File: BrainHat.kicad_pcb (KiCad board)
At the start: 2 copper layers, 86 x 51.2 mm, 47 parts, among them J1 Power, J2 Output, J3 Electrodes, J4 Status, U1 AD8232, U2 ADS1115IDGS, U3 TS5A3159ADBVR, U4 SN74LV1T34DBV, U5 SN74LV1T34DBV

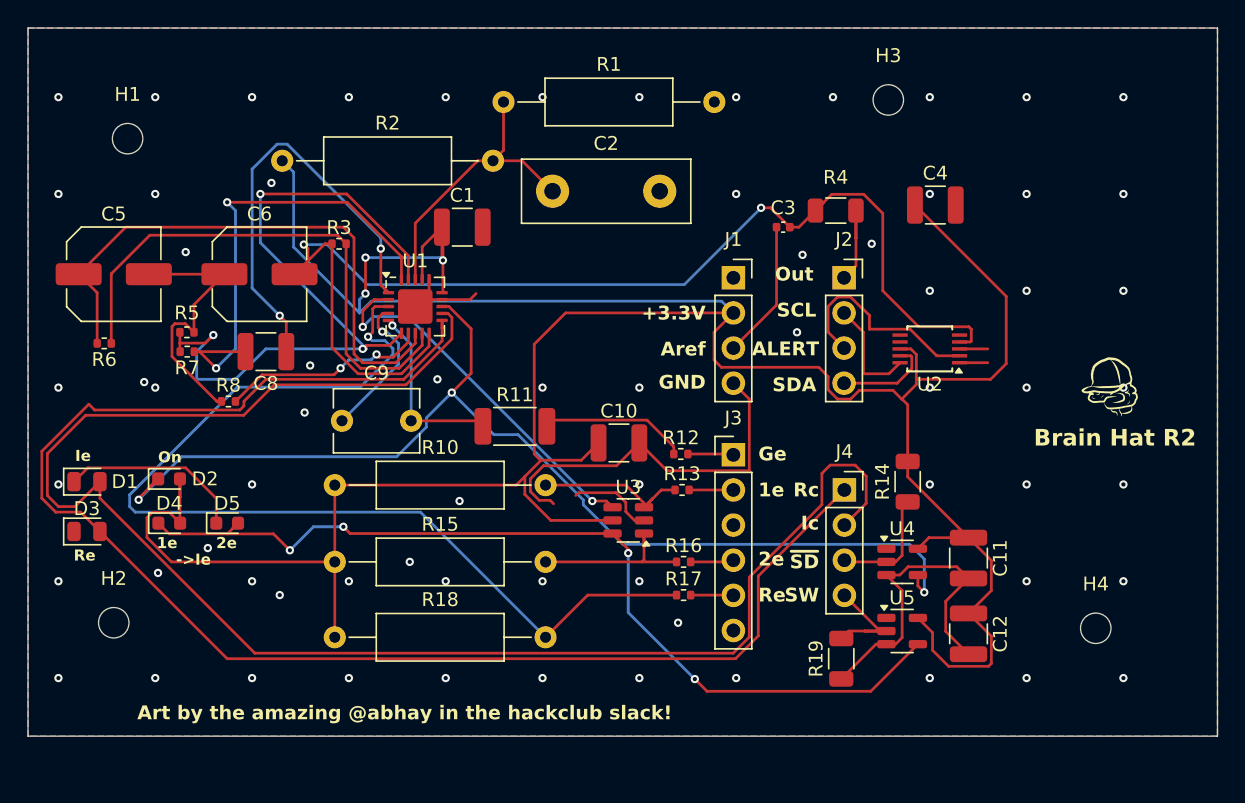
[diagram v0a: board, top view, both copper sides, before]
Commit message: Redid PCB again
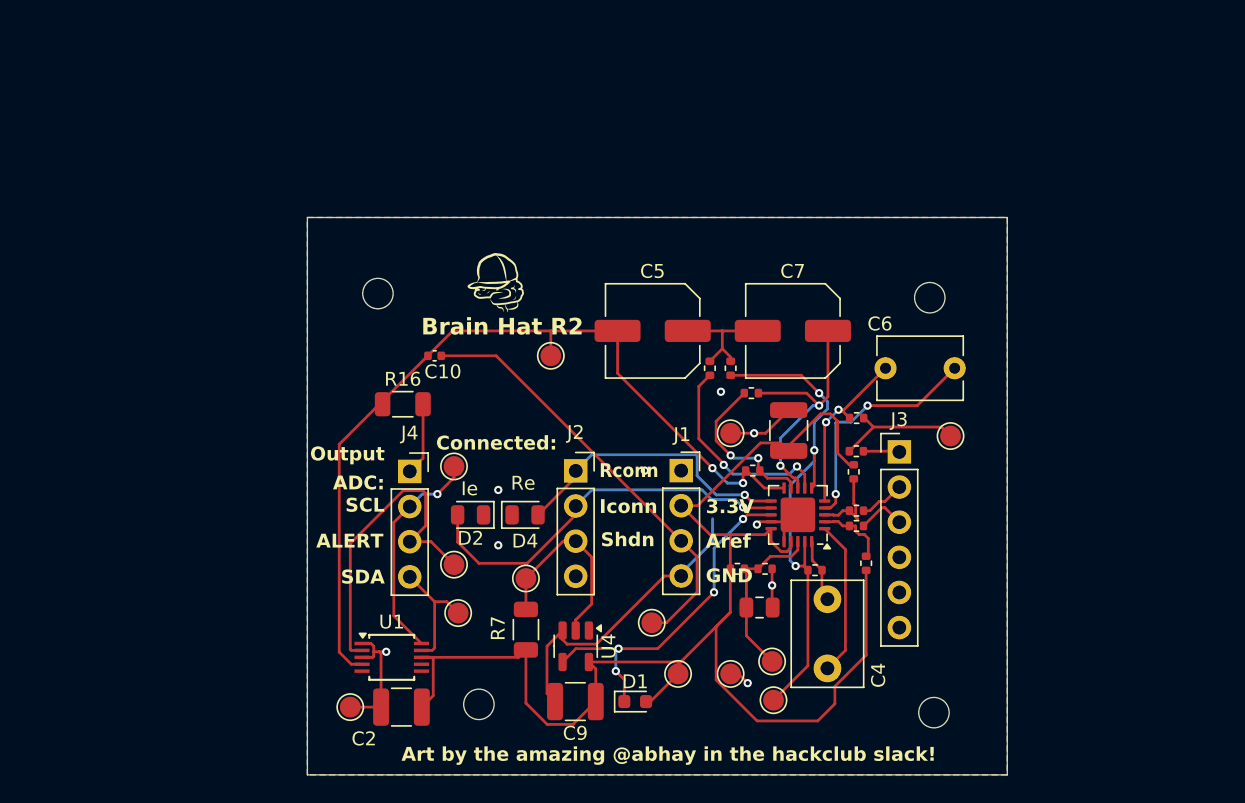
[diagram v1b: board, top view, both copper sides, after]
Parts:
- removed C11, C12, C8: 100nF, Capacitor_SMD:C_1210_3225Metric
- removed D3: XL-2012UWC, LED_SMD:LED_0805_2012Metric
- removed D5: XL-1608UGC-04, LED_SMD:LED_0603_1608Metric
- removed R17: 330k, Resistor_SMD:R_0402_1005Metric
- removed R18: 10M±1%, Resistor_THT:R_Axial_DIN0309_L9.0mm_D3.2mm_P15.24mm_Horizontal
- removed R19: 10k, Resistor_SMD:R_1206_3216Metric
- removed U3: TS5A3159ADBVR, Package_TO_SOT_SMD:SOT-23-6
- removed U5: SN74LV1T34DBV, Package_TO_SOT_SMD:SOT-23-5
- added C7: 220uF, Capacitor_SMD:C_Elec_6.3x5.4, F.Cu at (186.1, 72.9)
- added TP1: TestPoint, TestPoint:TestPoint_Pad_D1.5mm, F.Cu at (181.6, 80.3)
- added TP10: TestPoint, TestPoint:TestPoint_Pad_D1.5mm, F.Cu at (154.1, 100.1)
- added TP12: TestPoint, TestPoint:TestPoint_Pad_D1.5mm, F.Cu at (166.8, 90.8)
- added TP13: TestPoint, TestPoint:TestPoint_Pad_D1.5mm, F.Cu at (197.5, 80.5)
- added TP16: TestPoint, TestPoint:TestPoint_Pad_D1.5mm, F.Cu at (168.6, 74.7)
- added TP2: TestPoint, TestPoint:TestPoint_Pad_D1.5mm, F.Cu at (177.8, 97.7)
- added TP3: TestPoint, TestPoint:TestPoint_Pad_D1.5mm, F.Cu at (175.9, 94.0)
- added TP4: TestPoint, TestPoint:TestPoint_Pad_D1.5mm, F.Cu at (184.7, 99.6)
- added TP5: TestPoint, TestPoint:TestPoint_Pad_D1.5mm, F.Cu at (184.6, 96.8)
- added TP6: TestPoint, TestPoint:TestPoint_Pad_D1.5mm, F.Cu at (161.6, 89.8)
- added TP7: TestPoint, TestPoint:TestPoint_Pad_D1.5mm, F.Cu at (161.6, 82.7)
- added TP8: TestPoint, TestPoint:TestPoint_Pad_D1.5mm, F.Cu at (161.9, 93.3)
- added TP9: TestPoint, TestPoint:TestPoint_Pad_D1.5mm, F.Cu at (181.6, 97.7)
- C10: value 100nF -> 14pF; footprint Capacitor_SMD:C_1210_3225Metric -> Capacitor_SMD:C_0402_1005Metric
- C2: value 10nF -> 100nF; footprint Capacitor_THT:C_Disc_D12.0mm_W4.4mm_P7.75mm -> Capacitor_SMD:C_1210_3225Metric
- C3: value 14pF -> 10nF; footprint Capacitor_SMD:C_0402_1005Metric -> Capacitor_SMD:C_0805_2012Metric
- C4: footprint Capacitor_SMD:C_1210_3225Metric -> Capacitor_THT:C_Disc_D7.5mm_W5.0mm_P5.00mm
- C6: value 220uF -> 1nF; footprint Capacitor_SMD:C_Elec_6.3x5.4 -> Capacitor_THT:C_Disc_D6.0mm_W4.4mm_P5.00mm
- C9: value 1nF -> 100nF; footprint Capacitor_THT:C_Disc_D6.0mm_W4.4mm_P5.00mm -> Capacitor_SMD:C_1210_3225Metric
- D1: value XL-2012UWC -> XL-1608UBC-04; footprint LED_SMD:LED_0805_2012Metric -> LED_SMD:LED_0603_1608Metric
- D2: value XL-1608UBC-04 -> XL-2012UWC; footprint LED_SMD:LED_0603_1608Metric -> LED_SMD:LED_0805_2012Metric
- D4: value XL-1608UGC-04 -> XL-2012UWC; footprint LED_SMD:LED_0603_1608Metric -> LED_SMD:LED_0805_2012Metric
- J2: value Output -> Status
- J4: value Status -> Output
- R1, R15: footprint Resistor_THT:R_Axial_DIN0309_L9.0mm_D3.2mm_P15.24mm_Horizontal -> Resistor_SMD:R_0402_1005Metric
- R10: value 10M±1% -> 412k; footprint Resistor_THT:R_Axial_DIN0309_L9.0mm_D3.2mm_P15.24mm_Horizontal -> Resistor_SMD:R_0402_1005Metric
- R11: value 412k -> 1.2M; footprint Resistor_SMD:R_2010_5025Metric -> Resistor_SMD:R_0402_1005Metric
- R12: value 330k -> 1.2M
- R13: value 330k -> 1k
- R14: value 10k -> 10M±1%; footprint Resistor_SMD:R_1206_3216Metric -> Resistor_SMD:R_0402_1005Metric
- R16: value 330k -> 10k; footprint Resistor_SMD:R_0402_1005Metric -> Resistor_SMD:R_1206_3216Metric
- R2: value 10M±1% -> 1.58M; footprint Resistor_THT:R_Axial_DIN0309_L9.0mm_D3.2mm_P15.24mm_Horizontal -> Resistor_SMD:R_0402_1005Metric
- R3: value 604 -> 10M±1%
- R4: value 10k -> 330k; footprint Resistor_SMD:R_1206_3216Metric -> Resistor_SMD:R_0402_1005Metric
- R5: value 1.2M -> 330k
- R6: value 1k -> 330k
- R7: value 1.58M -> 10k; footprint Resistor_SMD:R_0402_1005Metric -> Resistor_SMD:R_1206_3216Metric
- R8: value 1.2M -> 604
- U1: value AD8232 -> ADS1115IDGS; footprint Package_CSP:LFCSP-20-1EP_4x4mm_P0.5mm_EP2.5x2.5mm -> Package_SO:TSSOP-10_3x3mm_P0.5mm
- U2: value ADS1115IDGS -> AD8232; footprint Package_SO:TSSOP-10_3x3mm_P0.5mm -> Package_CSP:LFCSP-20-1EP_4x4mm_P0.5mm_EP2.5x2.5mm
- moved H1 59.1 mm to (196.0, 70.5)
- moved R6 56.0 mm to (190.7, 87.0), turned to 0 degrees
- moved H3 52.8 mm to (163.4, 99.9)
- moved C6 50.7 mm to (197.8, 75.6), turned to 180 degrees
- moved R5 50.1 mm to (190.7, 85.9)
- moved R2 48.6 mm to (187.7, 90.2), turned to 180 degrees
- moved D1 42.7 mm to (174.7, 99.7)
- moved C5 39.2 mm to (176.0, 72.9), turned to 180 degrees
- moved C2 38.9 mm to (157.8, 100.1), turned to 180 degrees
- moved R3 38.7 mm to (184.1, 90.1)
- moved R8 38.2 mm to (183.2, 83.0)
- moved R15 38.1 mm to (190.5, 83.1), turned to -90 degrees
- moved R10 38.0 mm to (190.7, 79.2)
- moved R1 37.7 mm to (182.1, 90.1)
- moved C4 34.4 mm to (188.6, 97.3), turned to 90 degrees
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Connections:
- C10 pad 1: +3.3V -> Aref
- C10 pad 2: GND -> UFOUT1
- C2 pad 1: Vref -> +3.3V
- C3 pad 1: Aref -> Vref
- C3 pad 2: UFOUT1 -> GND
- C4 pad 1: +3.3V -> HPDRIVE1
- C4 pad 2: GND -> HPSENSE1
- C5 pad 1: REFOUT1 -> Net-(C5-Pad1)
- C5 pad 2: Net-(C5-Pad2) -> UFOUT1
- C6 pad 1: Net-(C5-Pad2) -> RLDFB1
- C6 pad 2: UFOUT1 -> RLD1
- C9 pad 1: RLDFB1 -> +3.3V
- C9 pad 2: RLD1 -> GND
- D1 pad 1: GND -> shutdown
- D1 pad 2: connectedI -> +3.3V
- D2 pad 1: shutdown -> GND
- D2 pad 2: +3.3V -> connectedI
- D4 pad 1: switch -> GND
- D4 pad 2: +3.3V -> connectedR
- J2 pad 1: 1o -> connectedR
- J2 pad 2: SCL -> connectedI
- J2 pad 3: ALERT -> 5Vshutdown
- J2 pad 4: SDA -> unconnected-(J2-Pin_4-Pad4)
- J3 pad 2: Net-(J3-Pin_2) -> /E-
- J3 pad 3: unconnected-(J3-Pin_3-Pad3) -> /E+
- J3 pad 4: Net-(J3-Pin_4) -> unconnected-(J3-Pin_4-Pad4)
- J3 pad 5: Net-(J3-Pin_5) -> unconnected-(J3-Pin_5-Pad5)
- J4 pad 1: connectedR -> 1o
- J4 pad 2: connectedI -> SCL
- J4 pad 3: 5Vshutdown -> ALERT
- J4 pad 4: 5Vswitch -> SDA
- R1 pad 1: Vref -> +3.3V
- R1 pad 2: GND -> Vref
- R10 pad 1: +3.3V -> RLD1
- R10 pad 2: 1e -> Ge
- R11 pad 1: RLD1 -> IAOUT1
- R11 pad 2: Ge -> Net-(C5-Pad1)
- R12 pad 1: Ge -> Net-(C5-Pad1)
- R12 pad 2: Net-(J3-Pin_1) -> OPAMP+1
- R13 pad 1: 1e -> OPAMP-1
- R13 pad 2: Net-(J3-Pin_2) -> REFOUT1
- R14 pad 1: 5Vshutdown -> +3.3V
- R14 pad 2: +3.3V -> IN+
- R15 pad 2: 2e -> IN-
- R16 pad 1: 2e -> 1o
- R16 pad 2: Net-(J3-Pin_4) -> UFOUT1
- R2 pad 1: +3.3V -> HPSENSE1
- R2 pad 2: Vref -> IAOUT1
- R3 pad 1: UFOUT1 -> Vref
- R3 pad 2: OPAMP-1 -> GND
- R4 pad 1: 1o -> Ge
- R4 pad 2: UFOUT1 -> Net-(J3-Pin_1)
- R5 pad 1: IAOUT1 -> IN-
- R5 pad 2: Net-(C5-Pad2) -> /E-
- R6 pad 1: OPAMP-1 -> IN+
- R6 pad 2: REFOUT1 -> /E+
- R7 pad 1: HPSENSE1 -> 5Vshutdown
- R7 pad 2: IAOUT1 -> +3.3V
- R8 pad 1: Net-(C5-Pad2) -> UFOUT1
- R8 pad 2: OPAMP+1 -> OPAMP-1
- U1 pad 1: HPDRIVE1 -> GND
- U1 pad 10: UFOUT1 -> SCL
- U1 pad 2: Ie -> ALERT
- U1 pad 3: Re -> GND
- U1 pad 4: RLDFB1 -> UFOUT1
- U1 pad 5: RLD1 -> unconnected-(U1-AIN1-Pad5)
- U1 pad 6: IAOUT1 -> unconnected-(U1-AIN2-Pad6)
- U1 pad 7: OPAMP+1 -> unconnected-(U1-AIN3-Pad7)
- U1 pad 8: REFOUT1 -> +3.3V
- U1 pad 9: OPAMP-1 -> SDA
- U2 pad 1: GND -> HPDRIVE1
- U2 pad 10: SCL -> UFOUT1
- U2 pad 2: ALERT -> IN+
- U2 pad 3: GND -> IN-
- U2 pad 4: UFOUT1 -> RLDFB1
- U2 pad 5: unconnected-(U2-AIN1-Pad5) -> RLD1
- U2 pad 6: unconnected-(U2-AIN2-Pad6) -> IAOUT1
- U2 pad 7: unconnected-(U2-AIN3-Pad7) -> OPAMP+1
- U2 pad 8: +3.3V -> REFOUT1
- U2 pad 9: SDA -> OPAMP-1
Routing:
- net +3.3V: track 230.0 -> 103.0 mm, vias 3 -> 0
- net connectedI: track 118.2 -> 28.4 mm, vias 0 -> 1
- net connectedR: track 108.7 -> 20.7 mm, vias 0 -> 1
- net Re: track 74.7 -> 0.00 mm, vias 1 -> 0
- net switch: track 67.1 -> 0.00 mm, vias 4 -> 0
- net shutdown: track 80.5 -> 25.5 mm, vias 3 -> 4
- net GND: track 80.3 -> 43.3 mm, vias 68 -> 9
- net HPSENSE1: track 34.1 -> 4.06 mm, vias 2 -> 0
- net Ie: track 27.8 -> 0.00 mm, vias 2 -> 0
- net OPAMP-1: track 38.9 -> 11.7 mm, vias 0 -> 2
- net UFOUT1: track 85.2 -> 62.0 mm
- net REFOUT1: track 41.6 -> 18.5 mm, vias 0 -> 2
- net Aref: track 10.0 -> 31.3 mm
- net HPDRIVE1: track 31.7 -> 11.3 mm, vias 2 -> 0
- net Net-(C5-Pad2): track 19.6 -> 0.00 mm
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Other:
- board size 86 x 51.2 mm -> 50.6 x 40.3 mm
- board text added: "3.3V"
- board text added: "ADC: SCL"
- board text added: "Connected:"
- board text added: "Iconn"
- board text added: "Output"
- board text added: "Rconn"
- board text added: "Shdn"
- board text removed: "+3.3V"
- board text removed: "->Ie"
- board text removed: "1e"
- board text removed: "2e"
- board text removed: "Ge"
- board text removed: "Ic"
- board text removed: "On"
- board text removed: "Out"
- board text removed: "Rc"
- board text removed: "SCL"
- board text removed: "SW"
- board text removed: "~{SD}"
